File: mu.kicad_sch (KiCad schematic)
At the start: 69 parts, among them J1 2060-1452/998-404, J2 Conn_02x03_Odd_Even, J3 USB_C_Receptacle_USB2.0_16P, J4 ESQ-110-14-G-D, U1 STM32F042F6P6, U10 TLV3603QDCKRQ1, U11 MICROFC-60035-SMT-TR1, U12 USBLC6-2SC6, U13 OPA656NB/250, U2 MAX5026EUT_T, U3 MCP4921-E/SN, U4 LM4040AIM3-2.5/NOPB, U5 W25Q128JVS, U6 TLV70433DBVT, U7 SN74LVC1G74DCUT, U8 sn65hvd230, U9 LT3045xDD

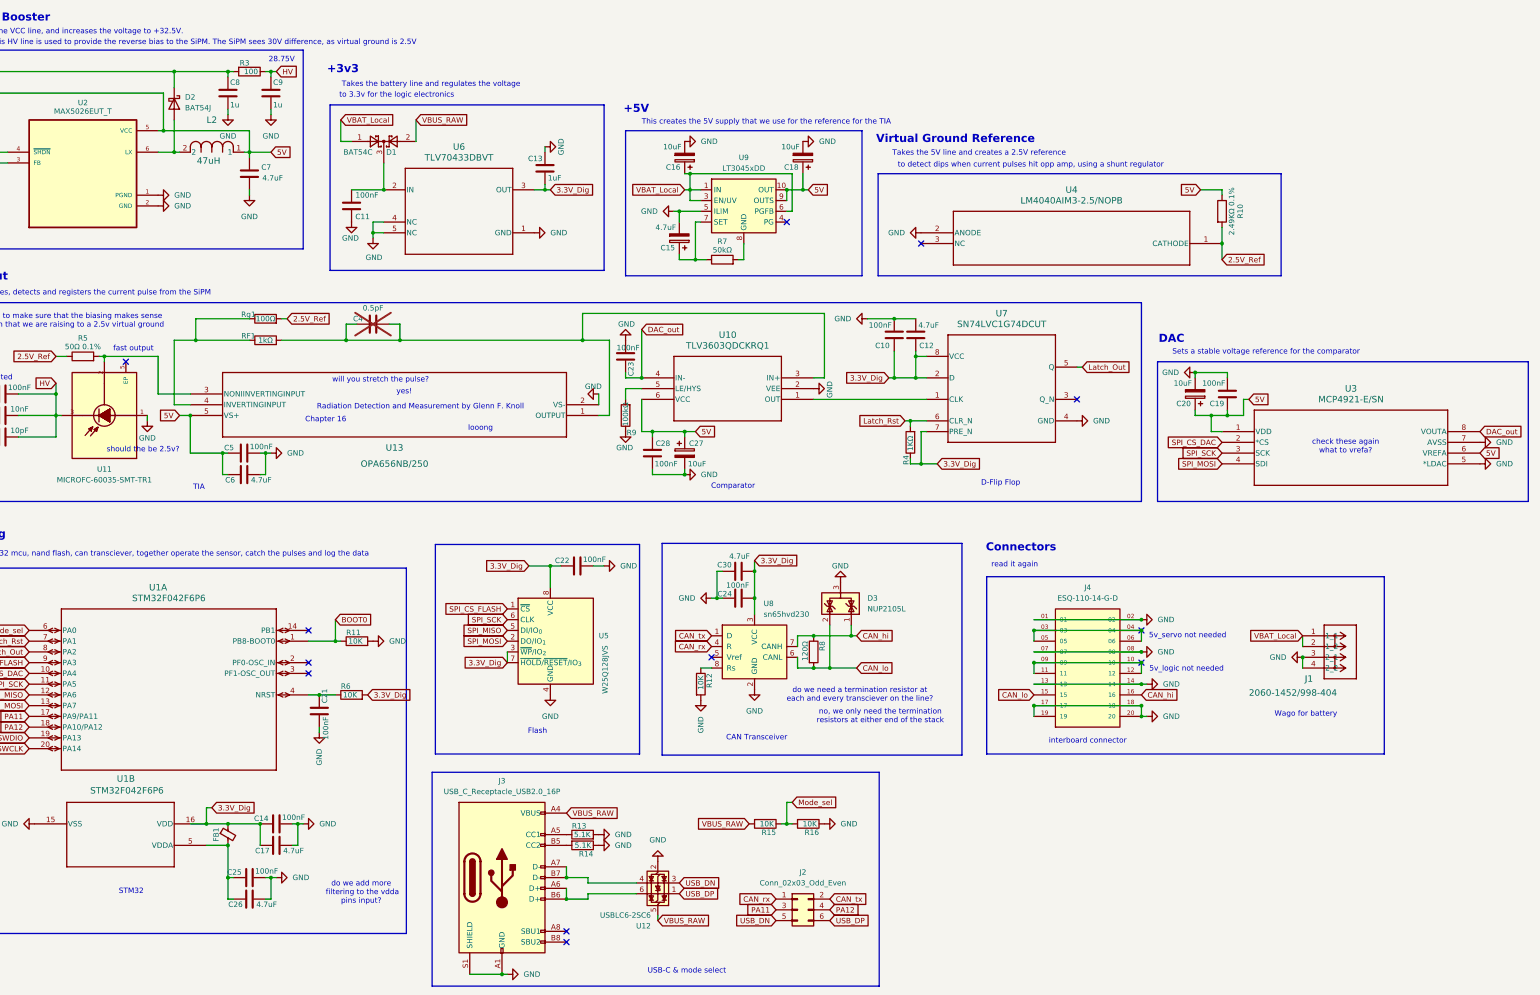
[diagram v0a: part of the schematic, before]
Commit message: ready to place
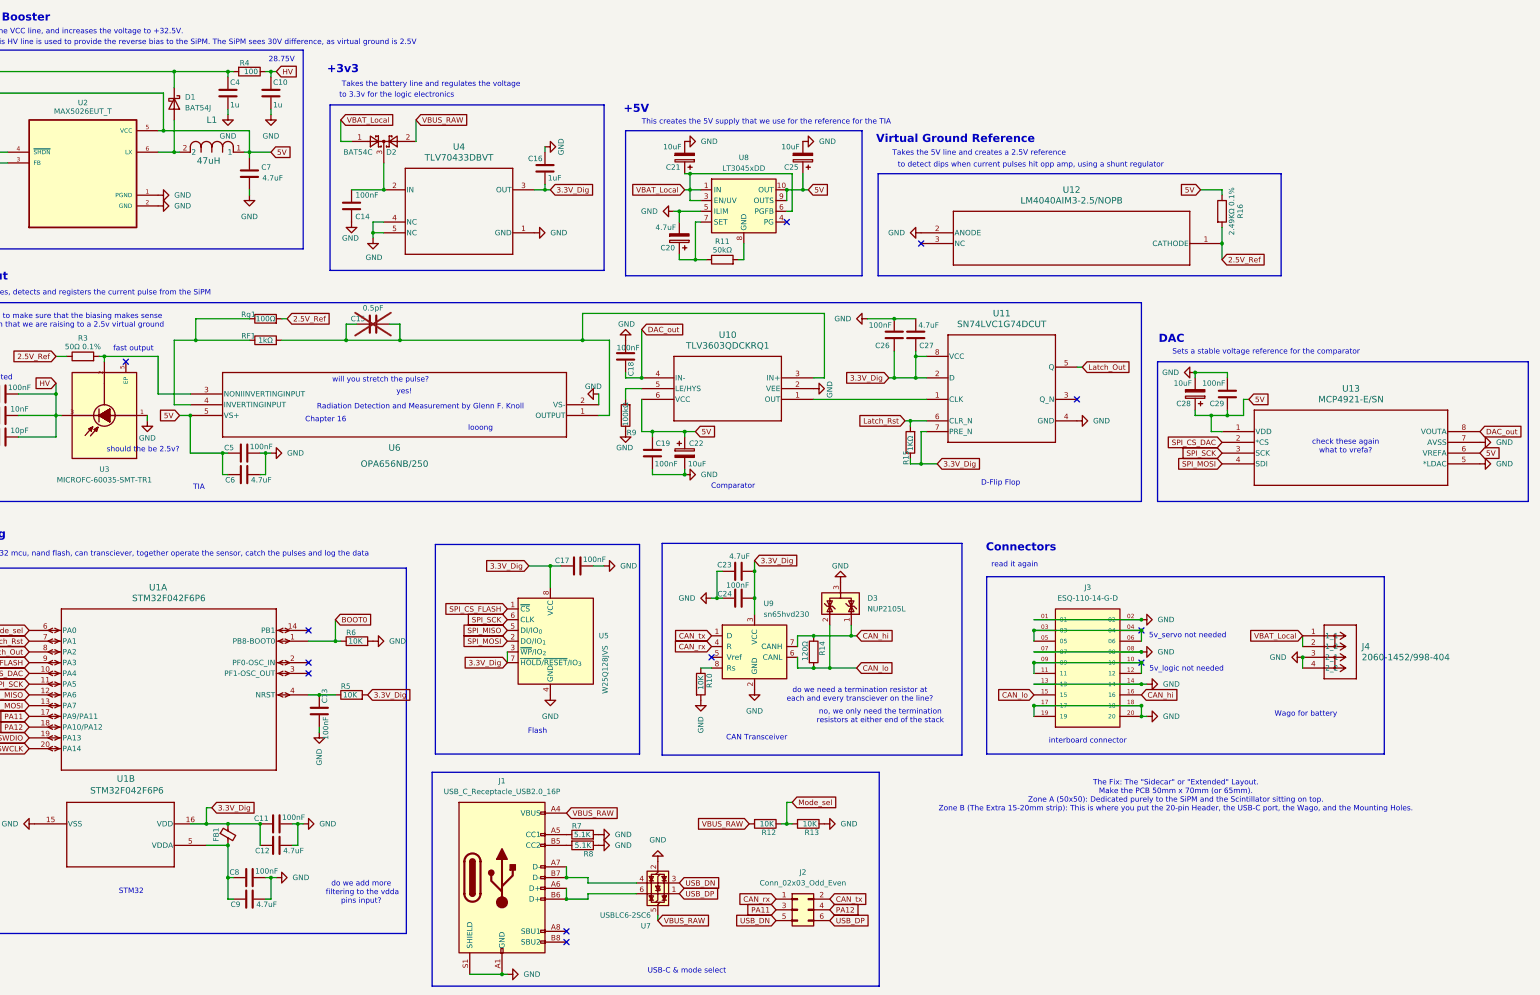
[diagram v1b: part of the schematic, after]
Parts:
- removed J1: 2060-1452/998-404, CONN2_2060-1452/998-404_WAG, symbol Wago 2060-1452 998-404:2060-1452_998-404
- added J4: 2060-1452/998-404, footprints:WAG, symbol Wago_2060-1452 998-404:2060-1452_998-404
- FB1: value ~ -> ferrite
- J3: renamed from J4; footprint ESQ-110-X-X-D:ESQ-110-X-X-D -> Connector_PinHeader_2.54mm:PinHeader_2x10_P2.54mm_Vertical
- renumbered C9 to C10, C14 to C11, C17 to C12, C21 to C13, C11 to C14, C4 to C15, C13 to C16, C22 to C17, C23 to C18, C28 to C19, C15 to C20, C16 to C21, C27 to C22, C30 to C23, C18 to C25, C10 to C26, C12 to C27, C20 to C28, C19 to C29, C8 to C4, C25 to C8, C26 to C9, D2 to D1, D1 to D2, J3 to J1, L2 to L1, R12 to R10, R7 to R11, R15 to R12, R16 to R13, R8 to R14, R4 to R15, R10 to R16, R5 to R3, R3 to R4, R6 to R5, R11 to R6, R13 to R7, R14 to R8, U7 to U11, U4 to U12, U3 to U13, U11 to U3, U6 to U4, U13 to U6, U12 to U7, U9 to U8, U8 to U9
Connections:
- net GND: now also J4.3 (2_1), J4.4 (2_2)
- net VBAT_Local: now also J4.1 (1_1), J4.2 (1_2)
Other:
- note added: "The Fix: The "Sidecar" or "Extended" Layout. Make the PCB 50mm x 70mm (or 65mm). Zone A (50x50): Dedicated purely to the SiPM and the Scintillator sitting on top. Zone B (The Extra 15-20mm strip): This is where you put the 20-pin Header, the USB-C port, the Wago, and the Mounting Holes."

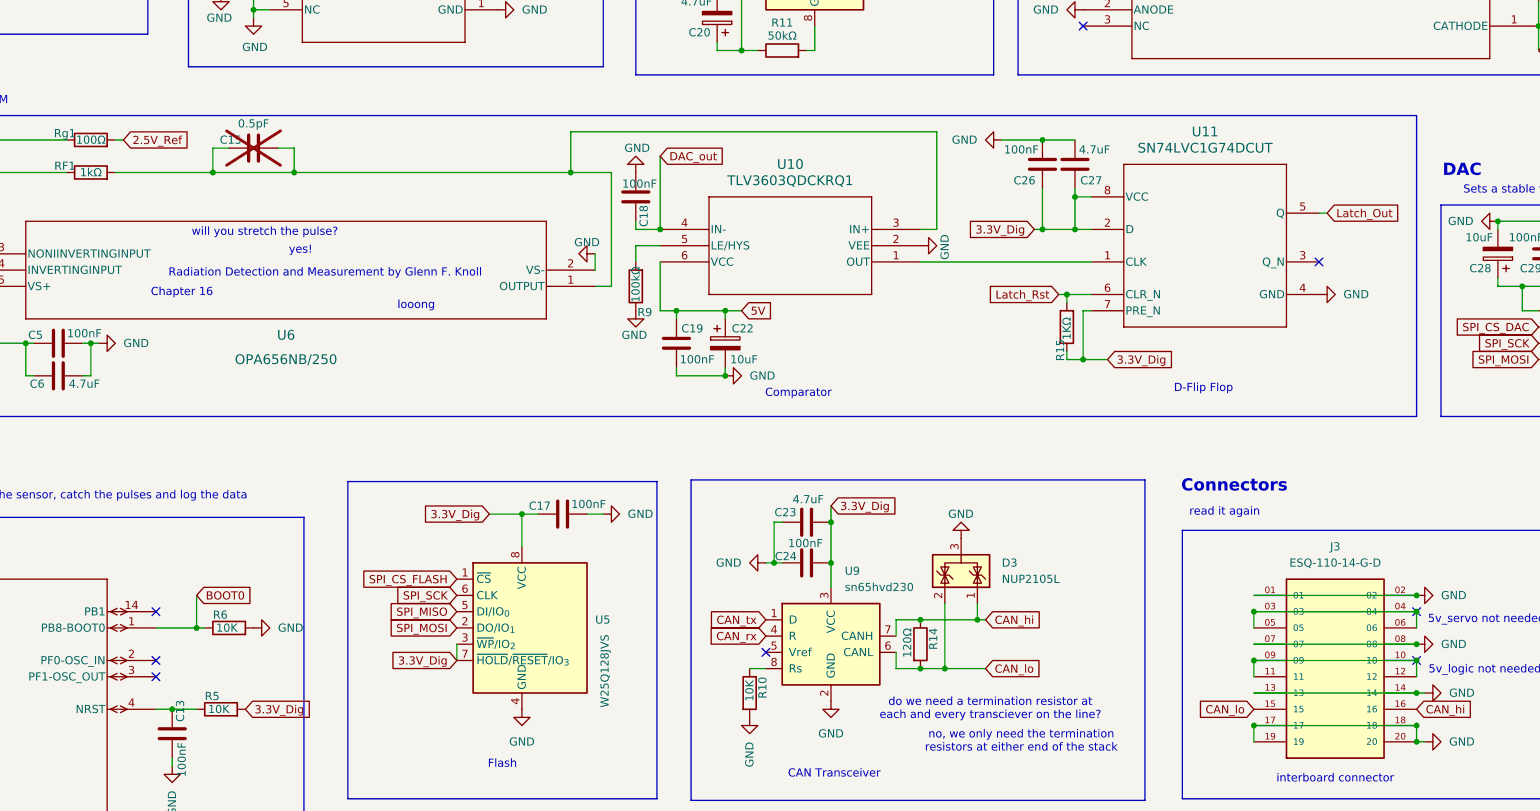
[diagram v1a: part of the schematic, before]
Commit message: O
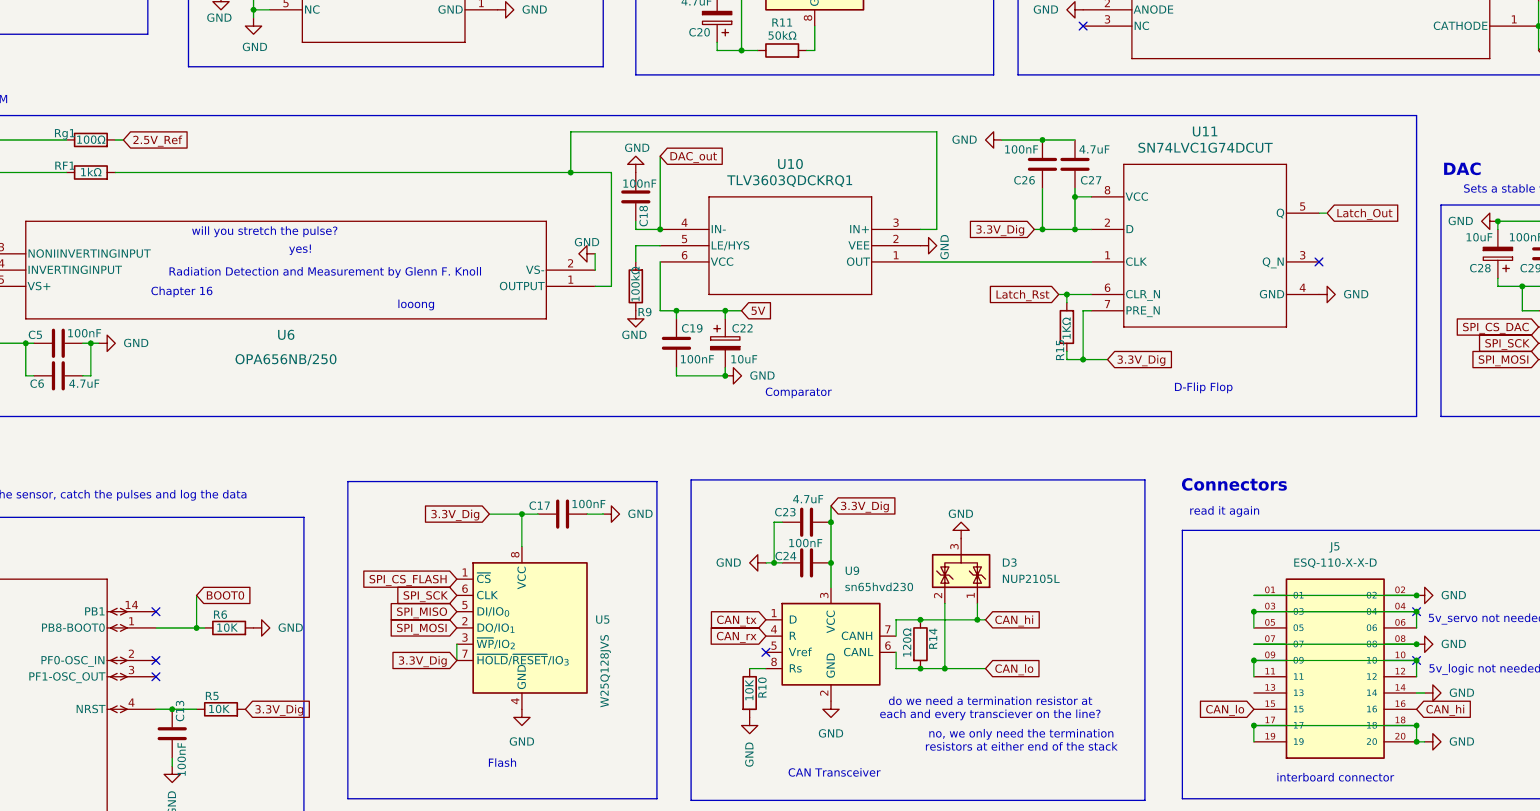
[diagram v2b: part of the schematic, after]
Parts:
- removed C15: 0.5pF, Capacitor_SMD:C_0402_1005Metric, symbol Device:C
- removed J3: ESQ-110-14-G-D, Connector_PinHeader_2.54mm:PinHeader_2x10_P2.54mm_Vertical, symbol ESQ-110-X-X-D:ESQ-110-X-X-D
- added J5: ESQ-110-X-X-D, SAMTEC_ESQ-110-14-G-D, symbol ESQ-110-X-X-D:ESQ-110-X-X-D
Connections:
- net CAN_hi: now also J5.16
- net CAN_lo: now also J5.15
- net GND: now also J5.01, J5.02, J5.07, J5.08, J5.14, J5.17, J5.18, J5.19, J5.20
- new net: J5.03, J5.04, J5.05, J5.06
- new net: J5.09, J5.10, J5.11, J5.12
